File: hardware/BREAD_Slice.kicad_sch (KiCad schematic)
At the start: 15 parts, among them J1 I2C_01x04, J2 Conn_01x10_Female

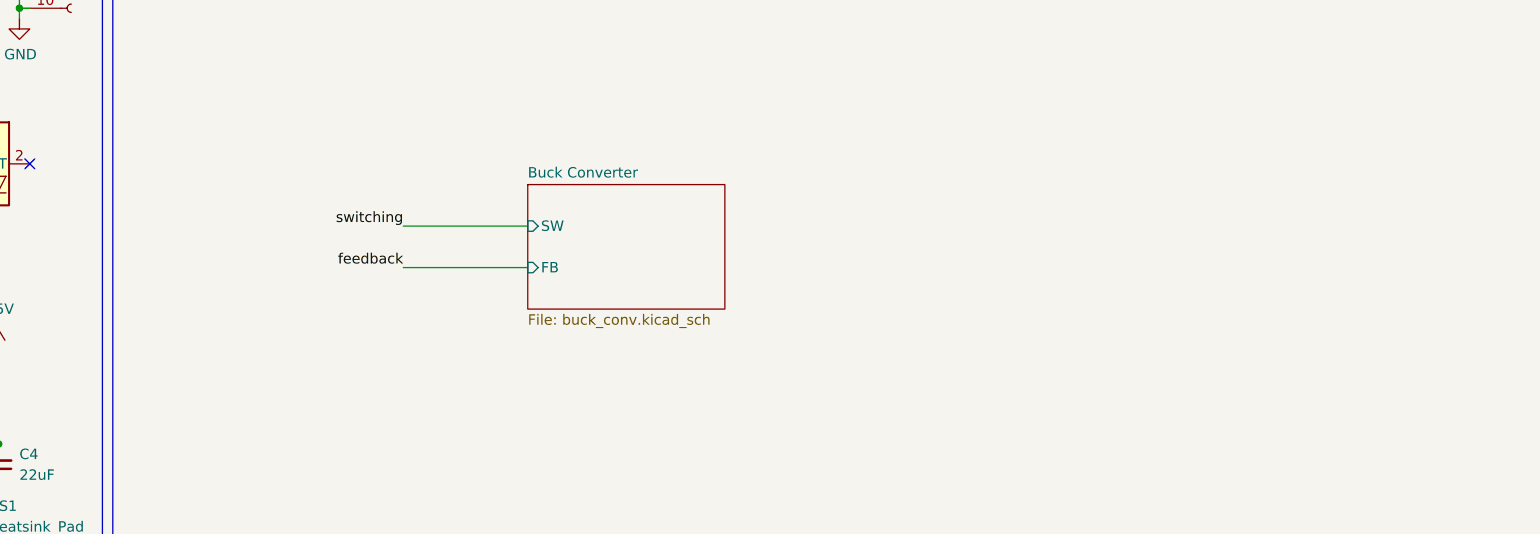
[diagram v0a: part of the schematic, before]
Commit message: JLCPCB order rev-A
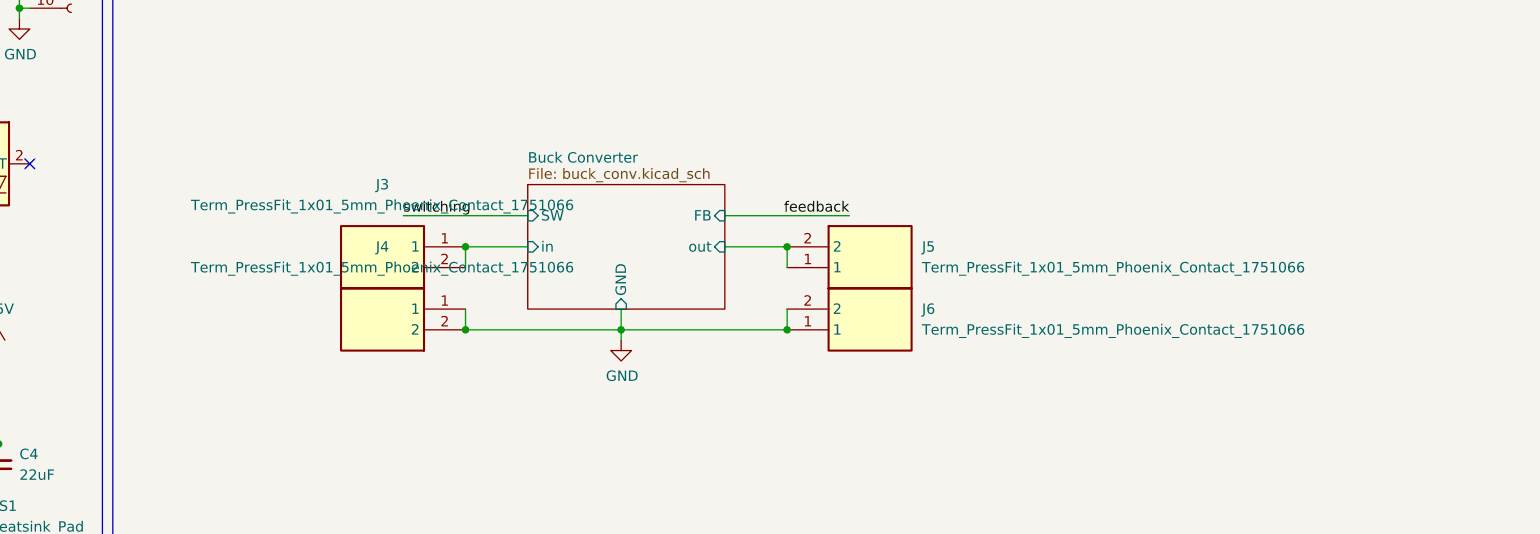
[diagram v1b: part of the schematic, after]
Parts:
- added J3, J4, J5, J6: Term_PressFit_1x01_5mm_Phoenix_Contact_1751066, KML-Custom:1751066, symbol kml-custom:Term_PressFit_1x01_5mm_Phoenix_Contact_1751066
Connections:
- net GND: now also J4.1, J4.2, J6.1, J6.2
- new net Buck Converter/in: J3.1, J3.2
- new net Buck Converter/out: J5.1, J5.2
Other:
- sheet Buck Converter ports: added GND, in, out; removed none
